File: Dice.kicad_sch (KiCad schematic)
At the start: 24 parts, among them Q1 NPN, SW1 SW_Push, U1 LM555xM, U2 4017, U3 74LS32

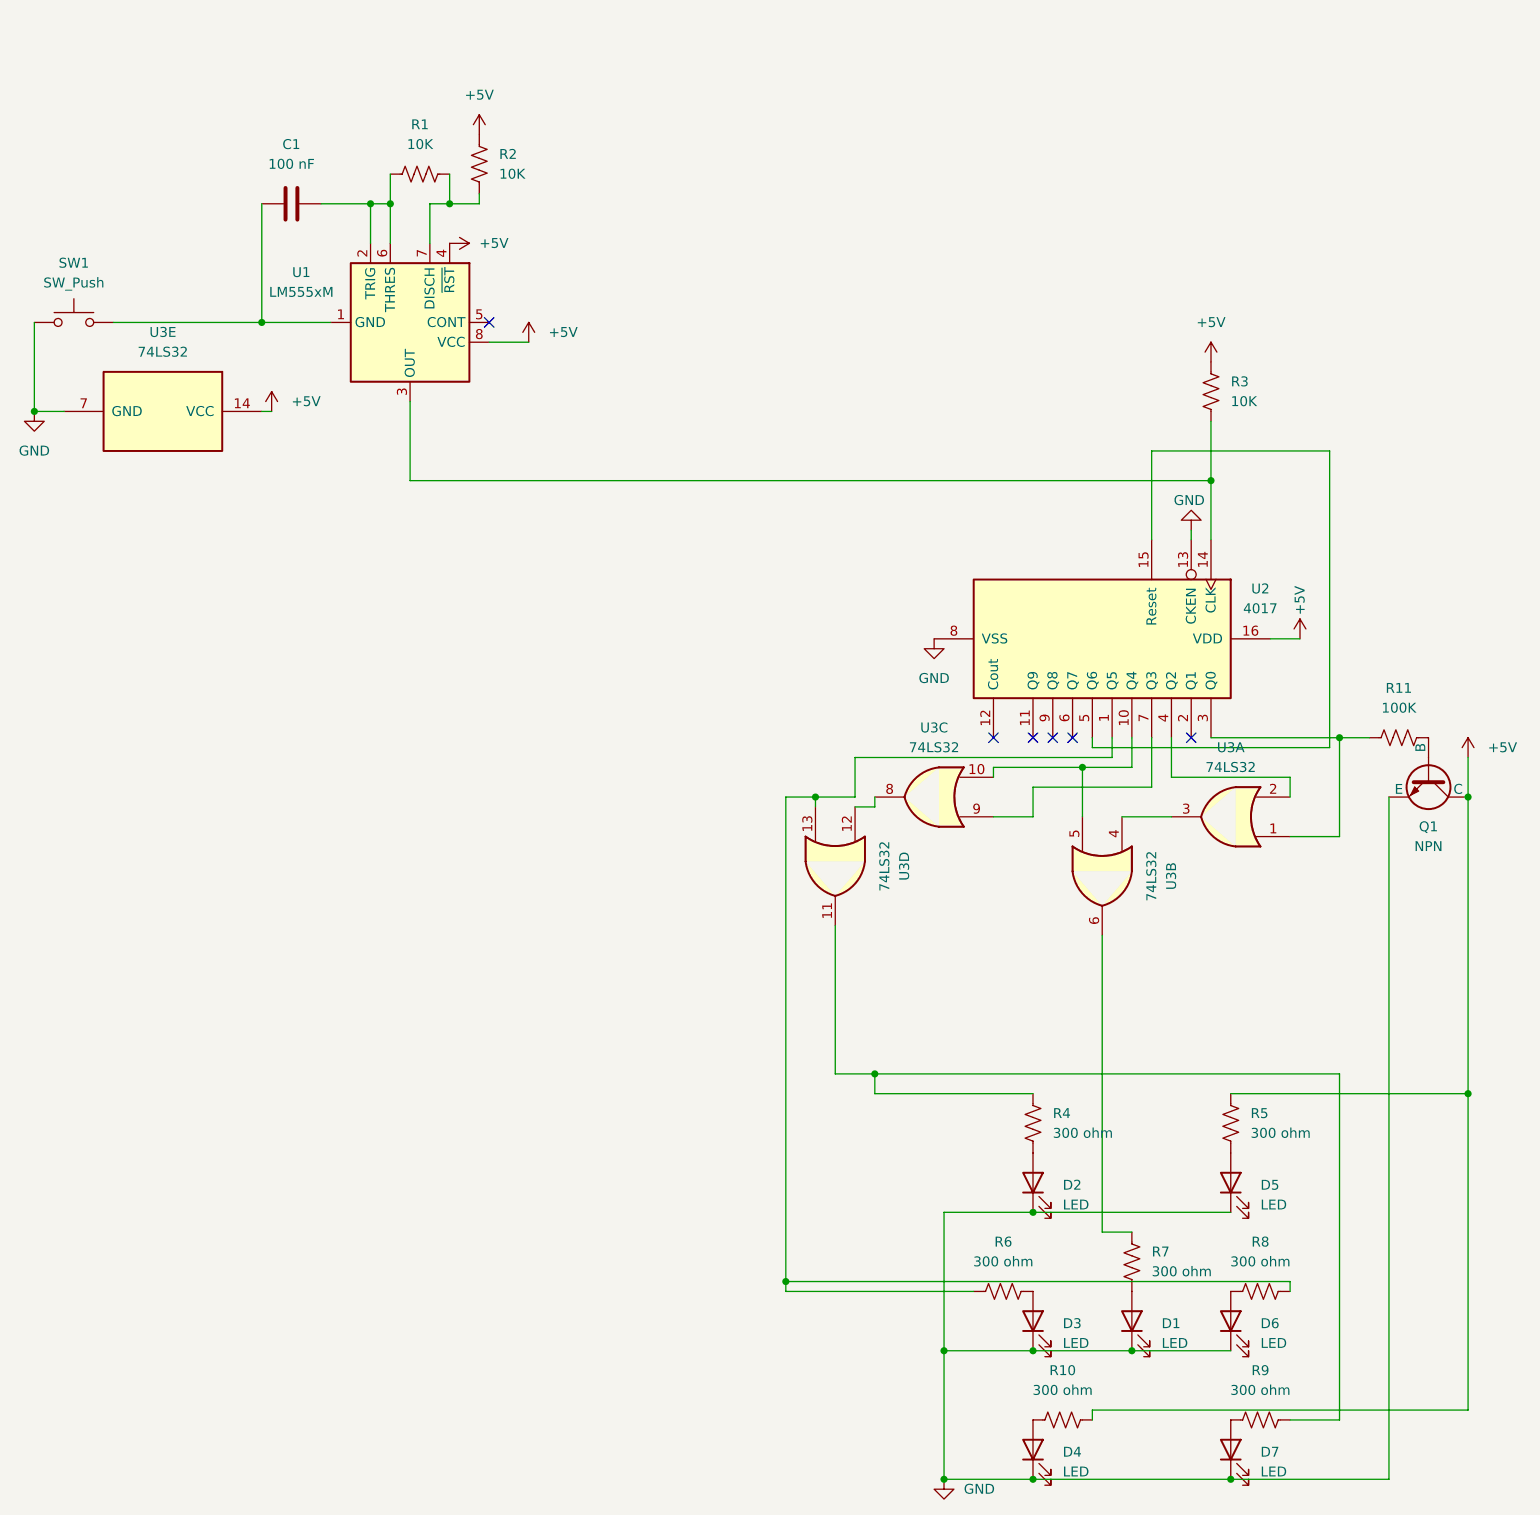
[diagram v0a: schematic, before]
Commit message: Test
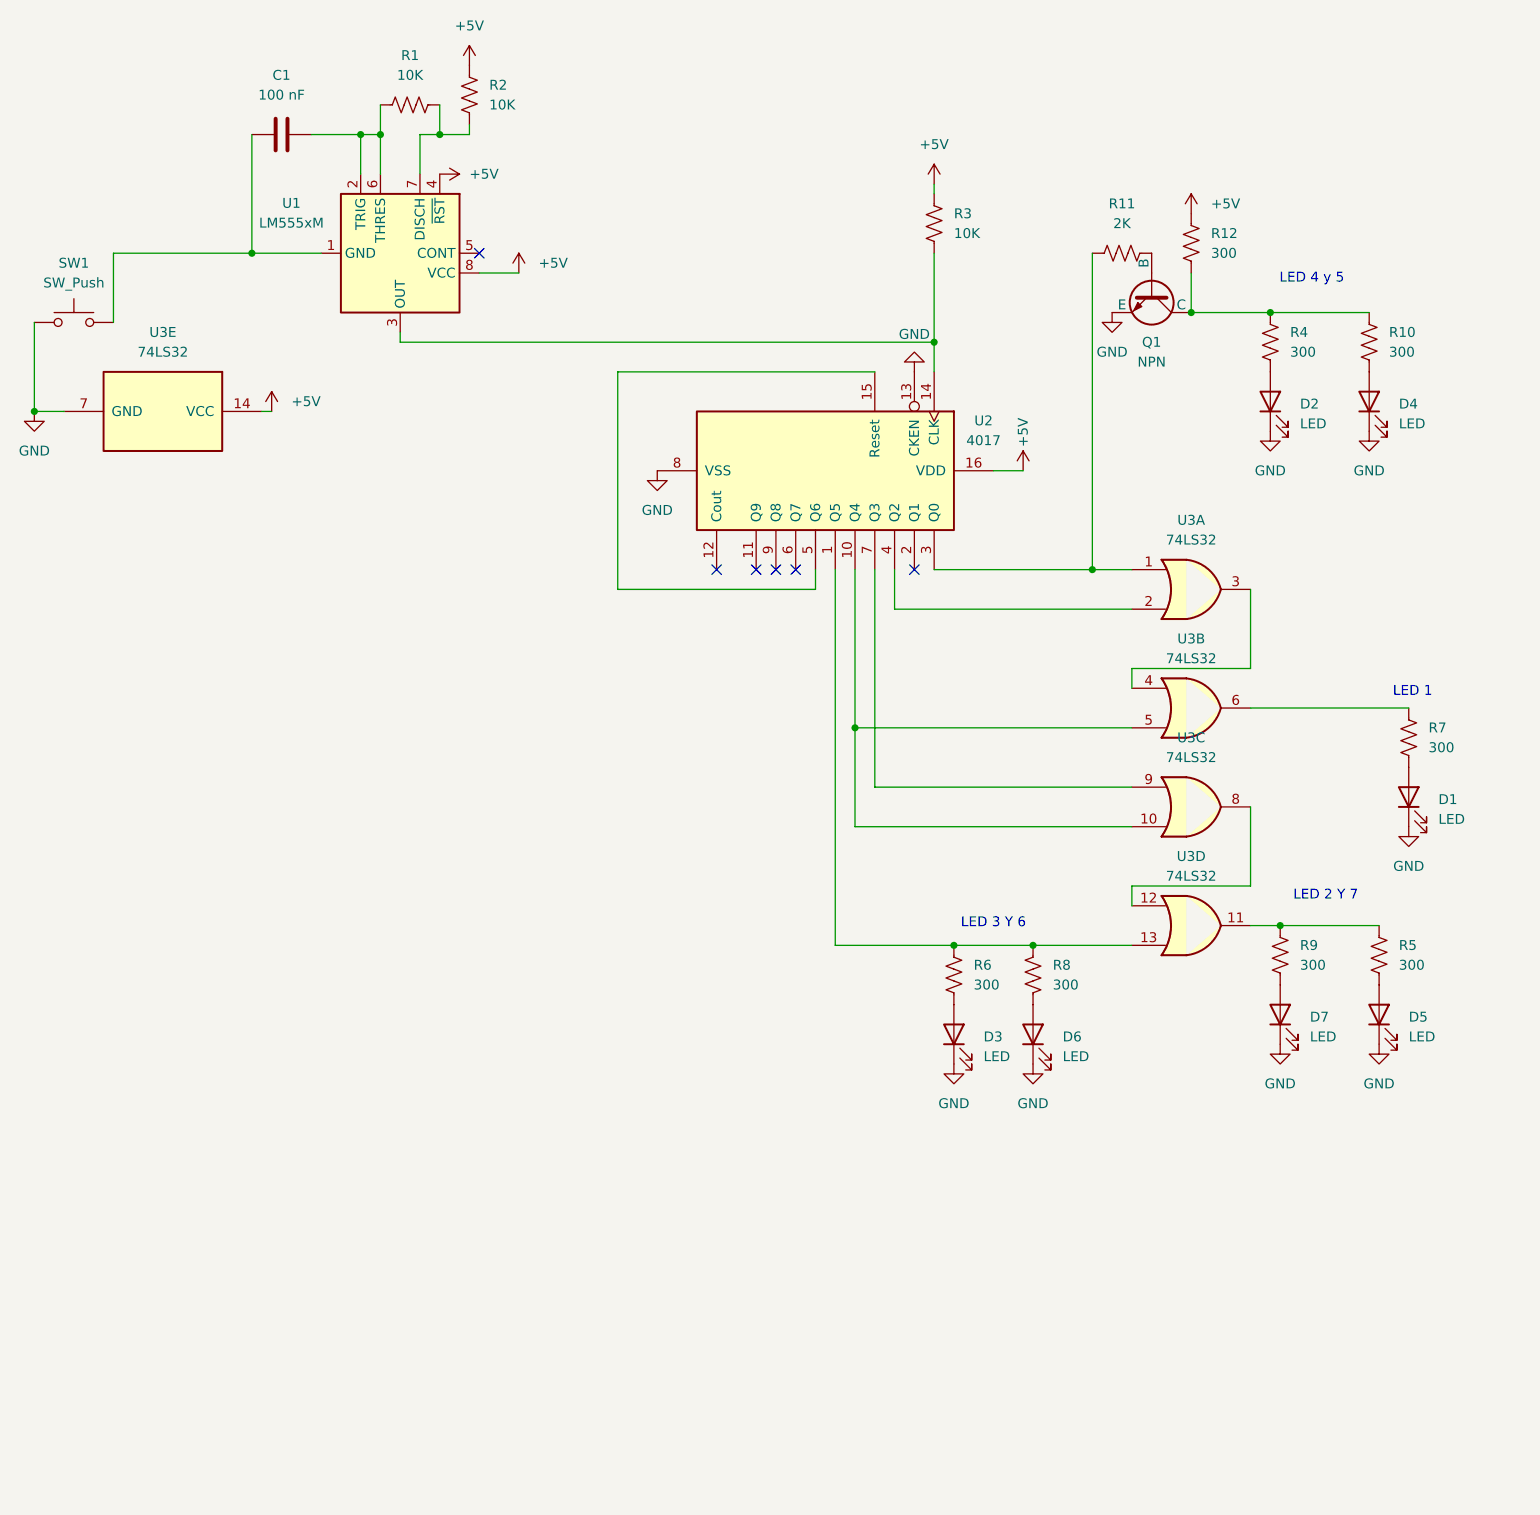
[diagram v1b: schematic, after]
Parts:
- added R12: 300, Package_DIP:DIP-8_W7.62mm, symbol Device:R_US
- R10, R4, R5, R6, R7, R8, R9: value 300 ohm -> 300
- R11: value 100K -> 2K
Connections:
- net +5V: now also R12.2; no longer Q1.1 (C), R10.1, R5.1
- net at R9.1, U3.11: now also R5.1; no longer R4.1
- net at R8.1, U2.1 (Q5), U3.13: now also R6.2; no longer R6.1
- net at D3.2 (A): now also R6.1; no longer R6.2
- new net: Q1.1 (C), R10.1, R12.1, R4.1
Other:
- note added: "LED 1"
- note added: "LED 2 Y 7"
- note added: "LED 3 Y 6"
- note added: "LED 4 y 5"
- moved on the sheet: C1, D1, D2, D3, D4, D5, D6, D7, Q1, R1, R10, R11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
